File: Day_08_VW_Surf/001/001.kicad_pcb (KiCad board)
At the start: 2 copper layers, 92.2 x 84.2 mm, 1 part

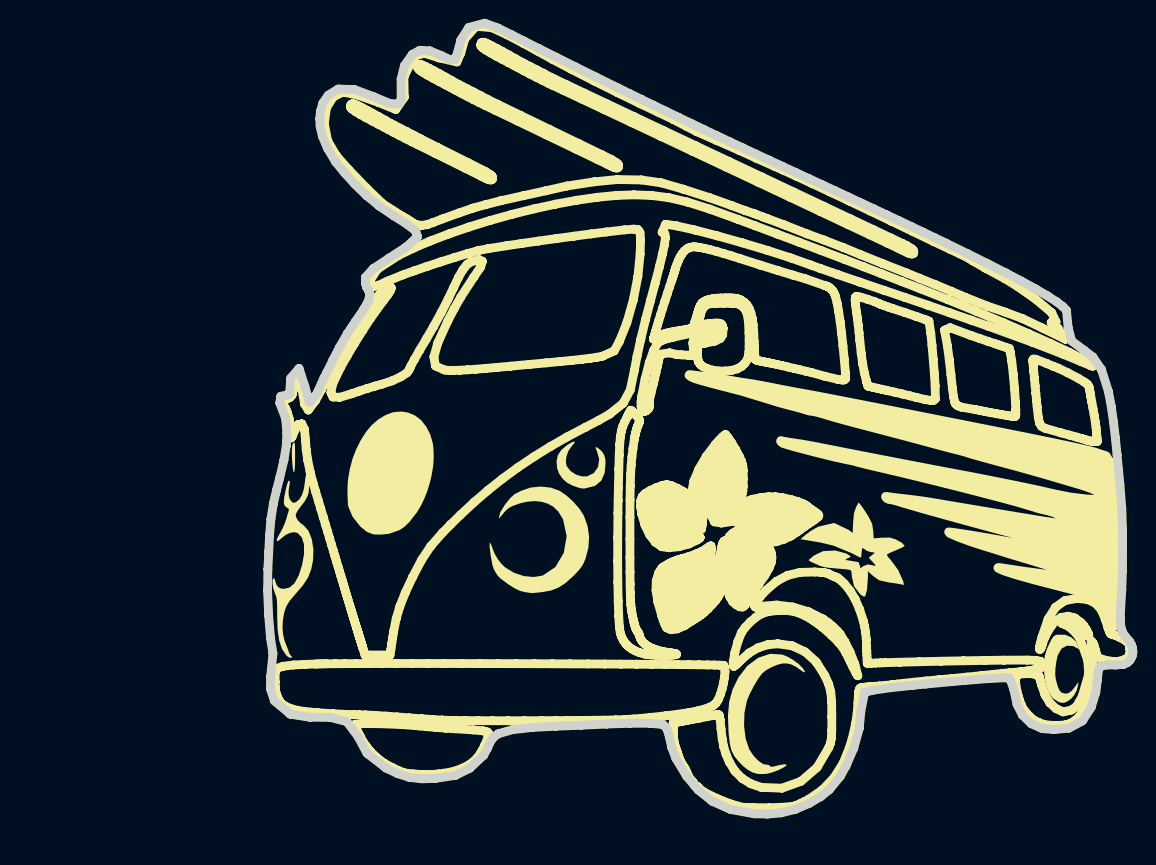
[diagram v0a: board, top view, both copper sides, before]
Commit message: Day 8 update
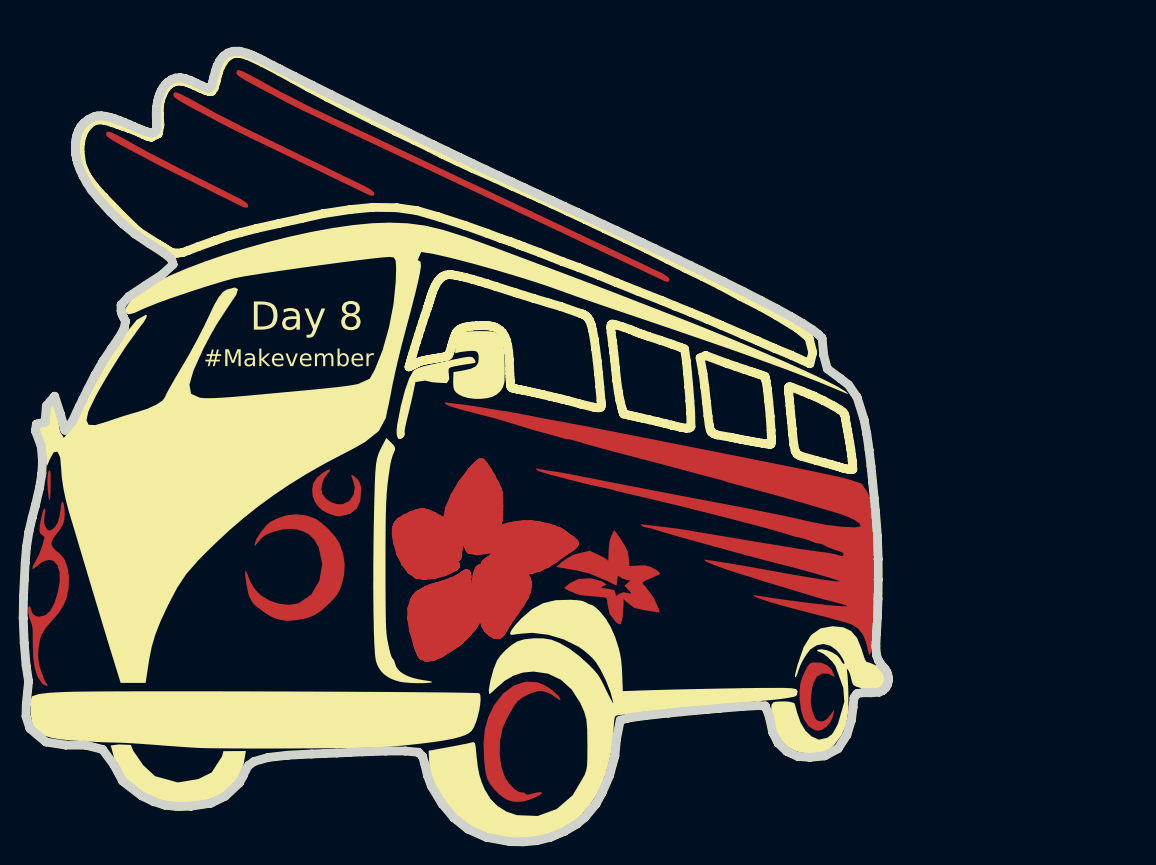
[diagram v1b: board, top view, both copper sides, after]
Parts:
- removed the svg2mod at (150.5, 94.6)
- added svg2mod: G***, combi:Combi.All.03, F.Cu at (124.5, 97.8)
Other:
- outline, holes or cut-outs redrawn
- board text added: "#Makevember"
- board text added: "Day 8"

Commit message: Update
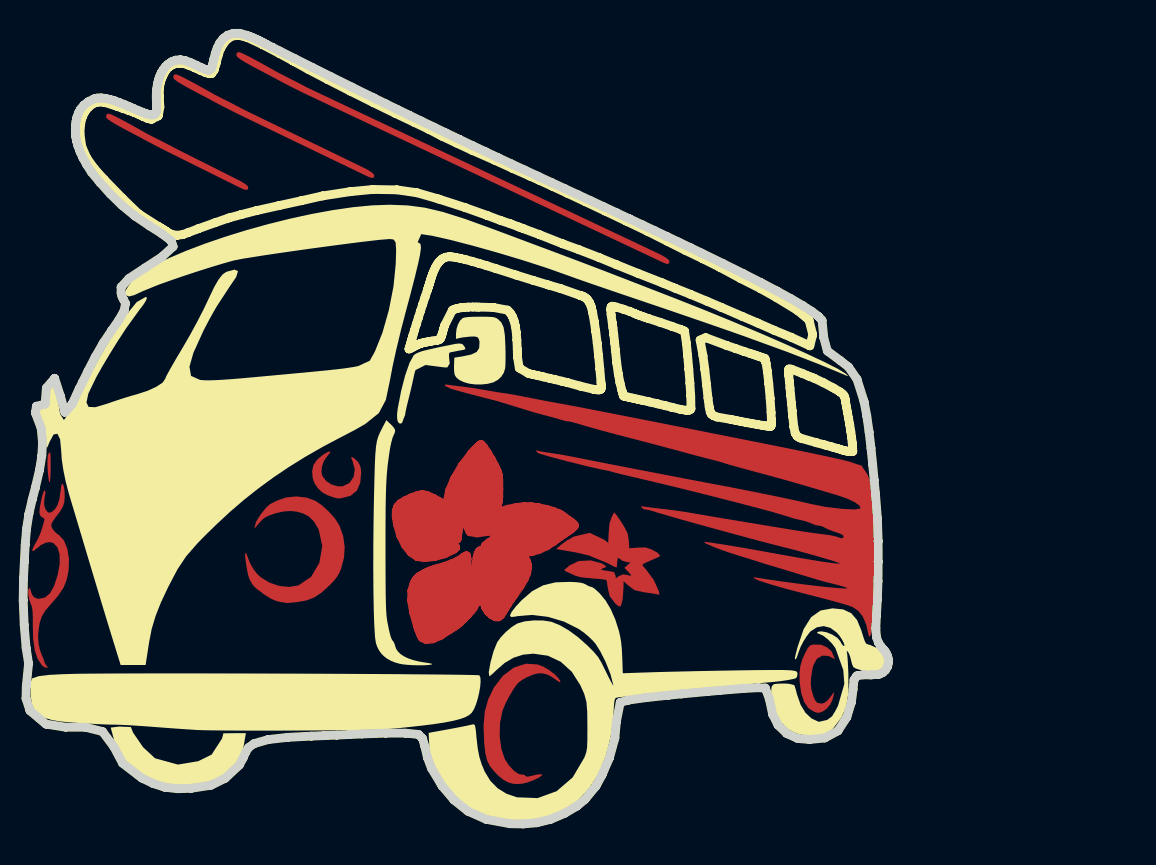
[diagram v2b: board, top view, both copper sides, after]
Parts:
- moved svg2mod 1.91 mm to (124.5, 95.9)
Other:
- board text removed: "#Makevember"
- board text removed: "Day 8"
